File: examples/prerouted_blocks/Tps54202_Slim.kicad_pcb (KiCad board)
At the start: 2 copper layers, 9 parts

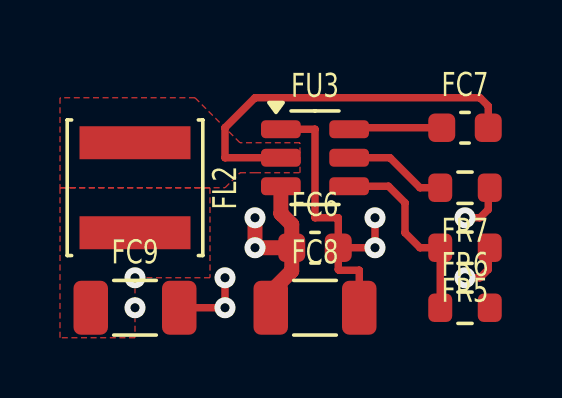
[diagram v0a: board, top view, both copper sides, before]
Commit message: wip converter layout
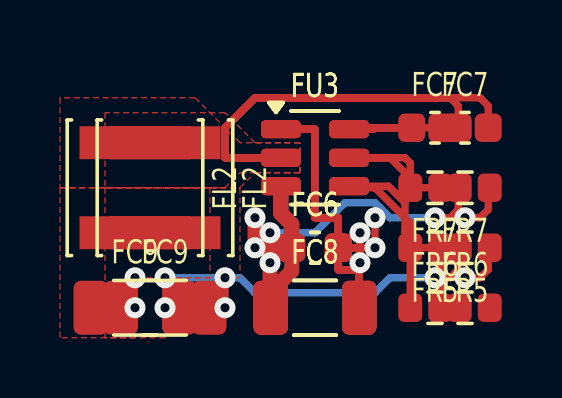
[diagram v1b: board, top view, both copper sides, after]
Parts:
- removed the FC6 at (68.0, 134.0)
- removed the FC8 at (68.0, 136.0)
- removed the FU3 at (68.0, 131.0)
- added FC6 (x2): reg_3v3.hf_in_cap, Capacitor_SMD:C_0603_1608Metric, F.Cu at (68.0, 134.0)
- added FC7: reg_3v3.boot_cap, Capacitor_SMD:C_0603_1608Metric, F.Cu at (72.0, 130.0)
- added FC8 (x2): reg_3v3.power_path.in_cap, Capacitor_SMD:C_1206_3216Metric, F.Cu at (68.0, 136.0)
- added FC9: reg_3v3.power_path.out_cap, Capacitor_SMD:C_1206_3216Metric, F.Cu at (63.0, 136.0)
- added FL2: reg_3v3.power_path.inductor, Inductor_SMD:L_Sunlord_SWPA4030S, F.Cu at (63.0, 132.0)
- added FR5: reg_3v3.fb.top_res, Resistor_SMD:R_0603_1608Metric, F.Cu at (72.0, 134.0)
- added FR6: reg_3v3.fb.bottom_res, Resistor_SMD:R_0603_1608Metric, F.Cu at (72.0, 136.0)
- added FR7: reg_3v3.en_res, Resistor_SMD:R_0603_1608Metric, F.Cu at (72.0, 132.0)
- added FU3 (x2): reg_3v3.ic, Package_TO_SOT_SMD:SOT-23-6, F.Cu at (68.0, 131.0)
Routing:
- net Fvin: track 7.80 -> 20.9 mm, vias 3 -> 6
- net Freg_3v3.ic.sw: track 12.9 -> 24.8 mm
- net Fv3v3: track 1.61 -> 12.6 mm, vias 3 -> 6
- net Fgnd: track 13.3 -> 24.1 mm, vias 4 -> 6
- net Freg_3v3.ic.fb: track 6.47 -> 12.0 mm
- net Freg_3v3.ic.en: track 3.45 -> 6.39 mm
- net Freg_3v3.ic.boot: track 3.04 -> 5.15 mm

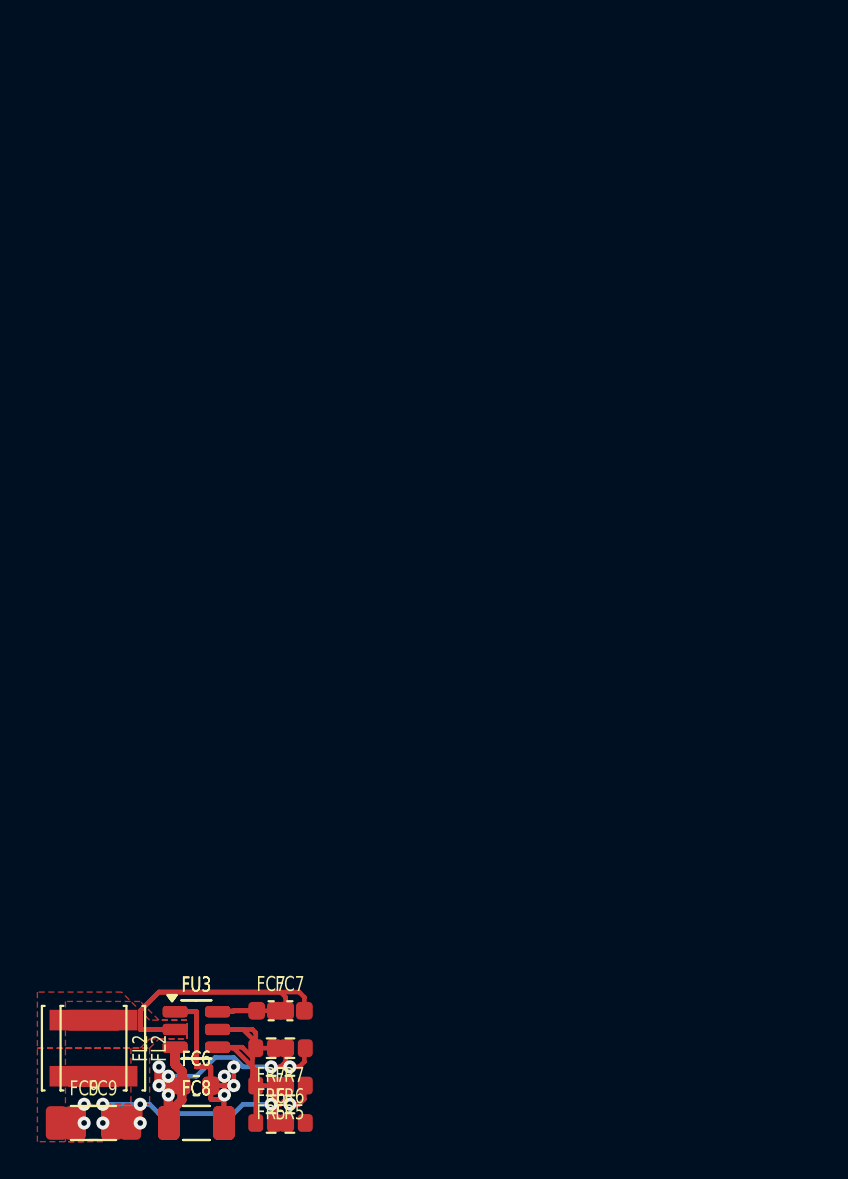
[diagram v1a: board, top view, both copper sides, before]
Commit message: layout wip
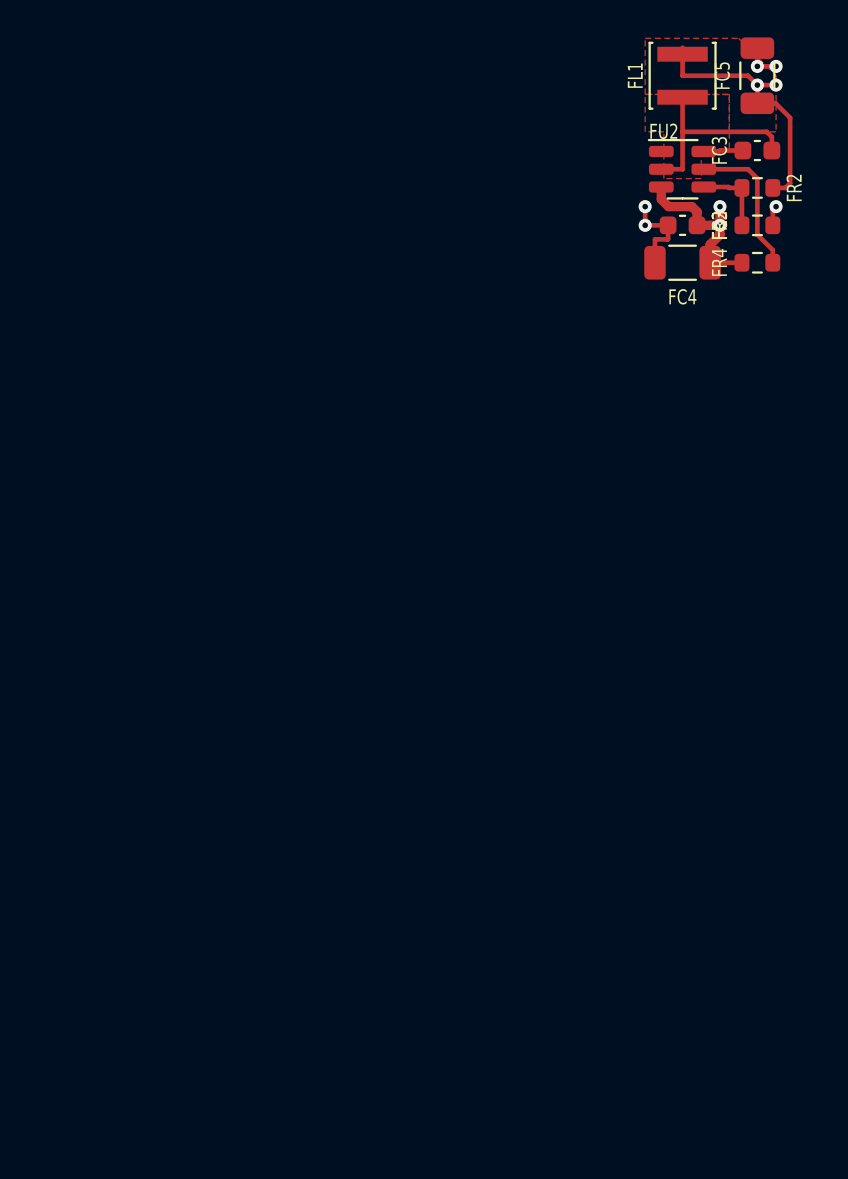
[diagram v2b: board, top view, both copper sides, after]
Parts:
- removed FC6 (x2): reg_3v3.hf_in_cap, Capacitor_SMD:C_0603_1608Metric
- removed FC7 (x2): reg_3v3.boot_cap, Capacitor_SMD:C_0603_1608Metric
- removed FC8 (x2): reg_3v3.power_path.in_cap, Capacitor_SMD:C_1206_3216Metric
- removed FC9 (x2): reg_3v3.power_path.out_cap, Capacitor_SMD:C_1206_3216Metric
- removed FL2 (x2): reg_3v3.power_path.inductor, Inductor_SMD:L_Sunlord_SWPA4030S
- removed FR5 (x2): reg_3v3.fb.top_res, Resistor_SMD:R_0603_1608Metric
- removed FR6 (x2): reg_3v3.fb.bottom_res, Resistor_SMD:R_0603_1608Metric
- removed FR7 (x2): reg_3v3.en_res, Resistor_SMD:R_0603_1608Metric
- removed FU3 (x2): reg_3v3.ic, Package_TO_SOT_SMD:SOT-23-6
- added FC2: reg_5v.hf_in_cap, Capacitor_SMD:C_0603_1608Metric, F.Cu at (94.0, 88.0)
- added FC3: reg_5v.boot_cap, Capacitor_SMD:C_0603_1608Metric, F.Cu at (98.0, 84.0)
- added FC4: reg_5v.power_path.in_cap, Capacitor_SMD:C_1206_3216Metric, F.Cu at (94.0, 90.0)
- added FC5: reg_5v.power_path.out_cap, Capacitor_SMD:C_1206_3216Metric, F.Cu at (98.0, 80.0)
- added FL1: reg_5v.power_path.inductor, Inductor_SMD:L_Sunlord_SWPA3015S, F.Cu at (94.0, 80.0)
- added FR2: reg_5v.fb.top_res, Resistor_SMD:R_0603_1608Metric, F.Cu at (98.0, 86.0)
- added FR3: reg_5v.fb.bottom_res, Resistor_SMD:R_0603_1608Metric, F.Cu at (98.0, 88.0)
- added FR4: reg_5v.en_res, Resistor_SMD:R_0603_1608Metric, F.Cu at (98.0, 90.0)
- added FU2: reg_5v.ic, Package_TO_SOT_SMD:SOT-23-6, F.Cu at (94.0, 85.0)
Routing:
- net Freg_3v3.ic.sw: track 24.8 -> 0.00 mm
- net Fgnd: track 24.1 -> 7.96 mm, vias 6 -> 5
- net Fv5: track 0.00 -> 14.3 mm, vias 0 -> 2
- net Fv3v3: track 12.6 -> 0.00 mm, vias 6 -> 0
- net Freg_3v3.ic.fb: track 12.0 -> 0.00 mm
- net Fvin: track 20.9 -> 9.72 mm, vias 6 -> 2
- net Freg_5v.ic.sw: track 0.00 -> 10.3 mm
- net Freg_5v.ic.en: track 0.00 -> 7.91 mm
- net Freg_3v3.ic.en: track 6.39 -> 0.00 mm
- net Freg_3v3.ic.boot: track 5.15 -> 0.00 mm
- net Freg_5v.ic.fb: track 0.00 -> 4.06 mm
- net Freg_5v.ic.boot: track 0.00 -> 2.11 mm
- added copper zone on F.Cu, net Freg_5v.ic.sw
- added copper zone on F.Cu, net Fv5
- removed copper zone on F.Cu, net Freg_3v3.ic.sw
- removed copper zone on F.Cu, net Fv3v3
